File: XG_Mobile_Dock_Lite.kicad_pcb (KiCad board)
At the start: 4 copper layers, 220 x 65 mm, 58 parts, among them J1 5-1775443-8, J10 SWD, J11 UART, J12 I2C1, J13 39300240, J14 469911008, J2 20455-040E-76, J3 20455-040E-76, J4 3-2362375-4, J5 USB_C_Receptacle, Q16 AO3401A, Q17 2N7002W, SW1 SW_Push, U12 STM32F030C8Tx

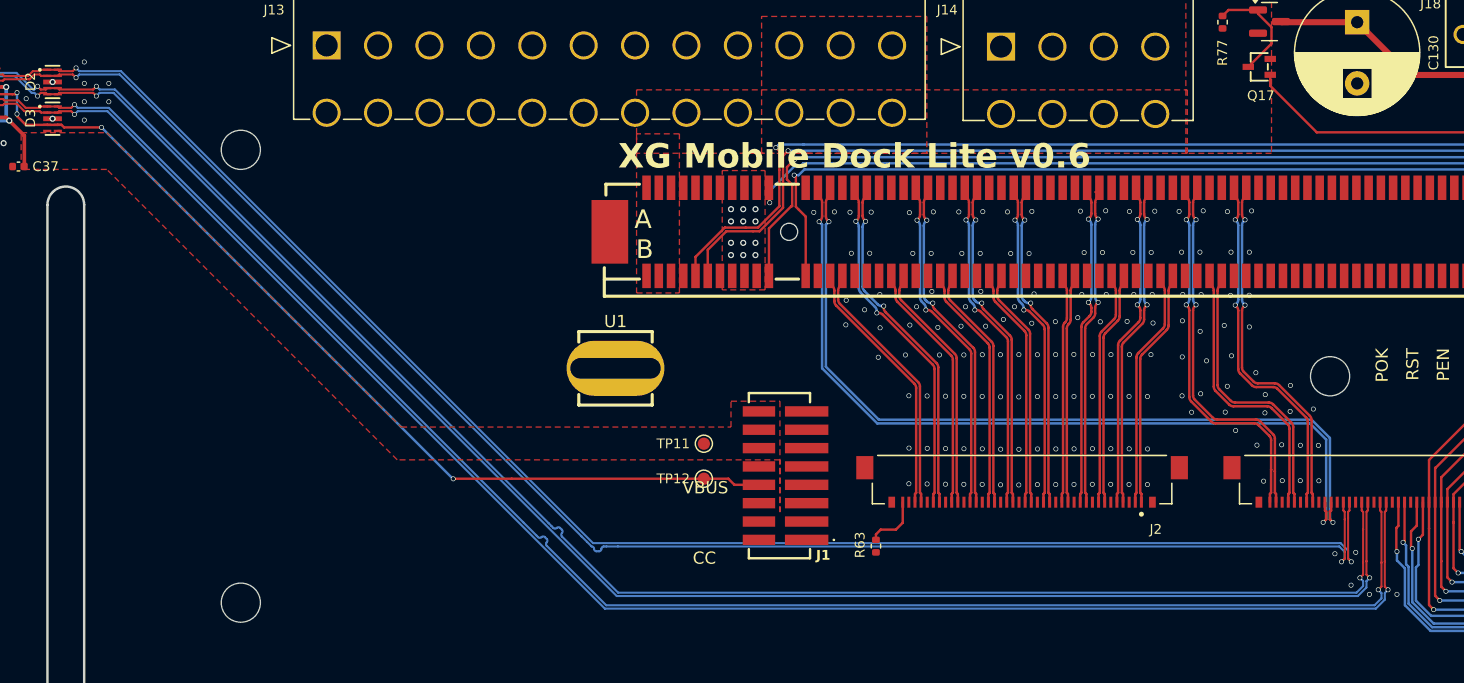
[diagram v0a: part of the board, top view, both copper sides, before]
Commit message: mroe tweaks
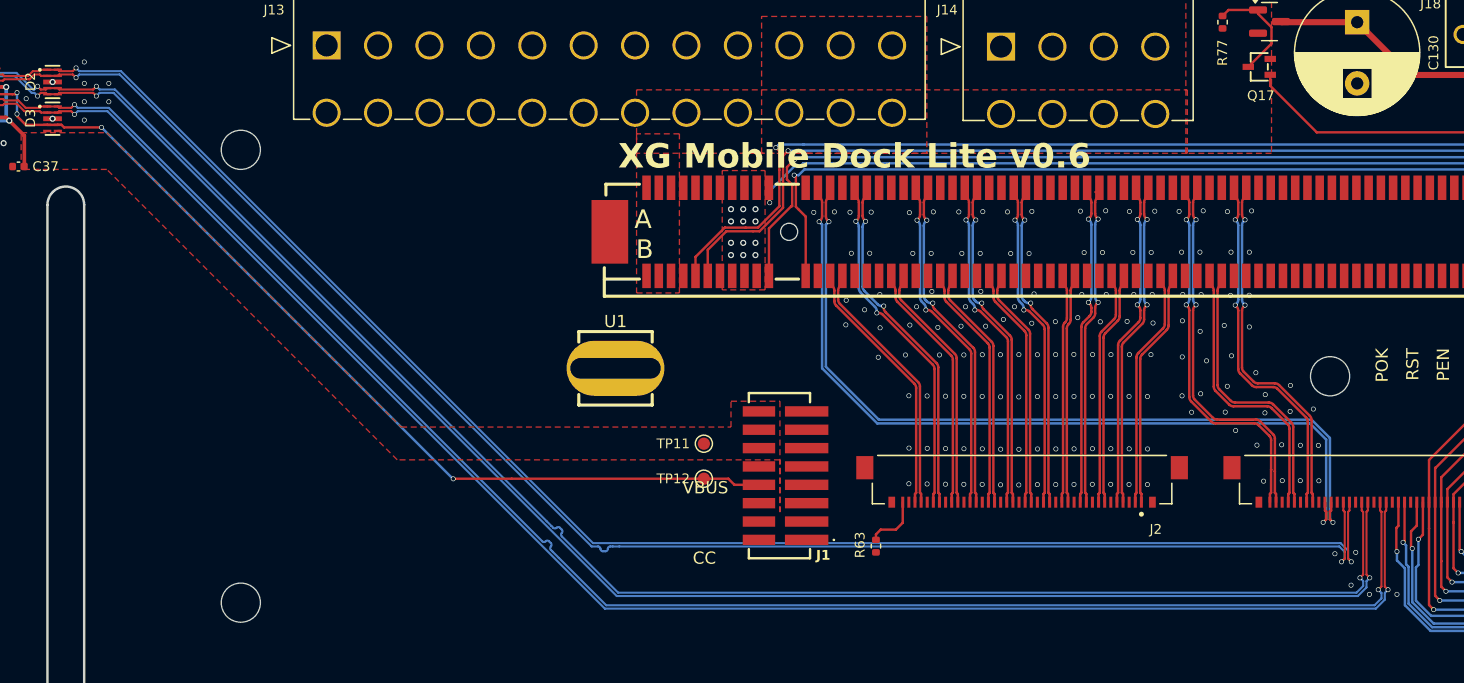
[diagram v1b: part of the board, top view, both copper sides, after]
